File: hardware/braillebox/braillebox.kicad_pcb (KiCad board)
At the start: 2 copper layers, 30 x 30 mm, 1 part, among them U1 XIAO-ESP32-S3-DIP

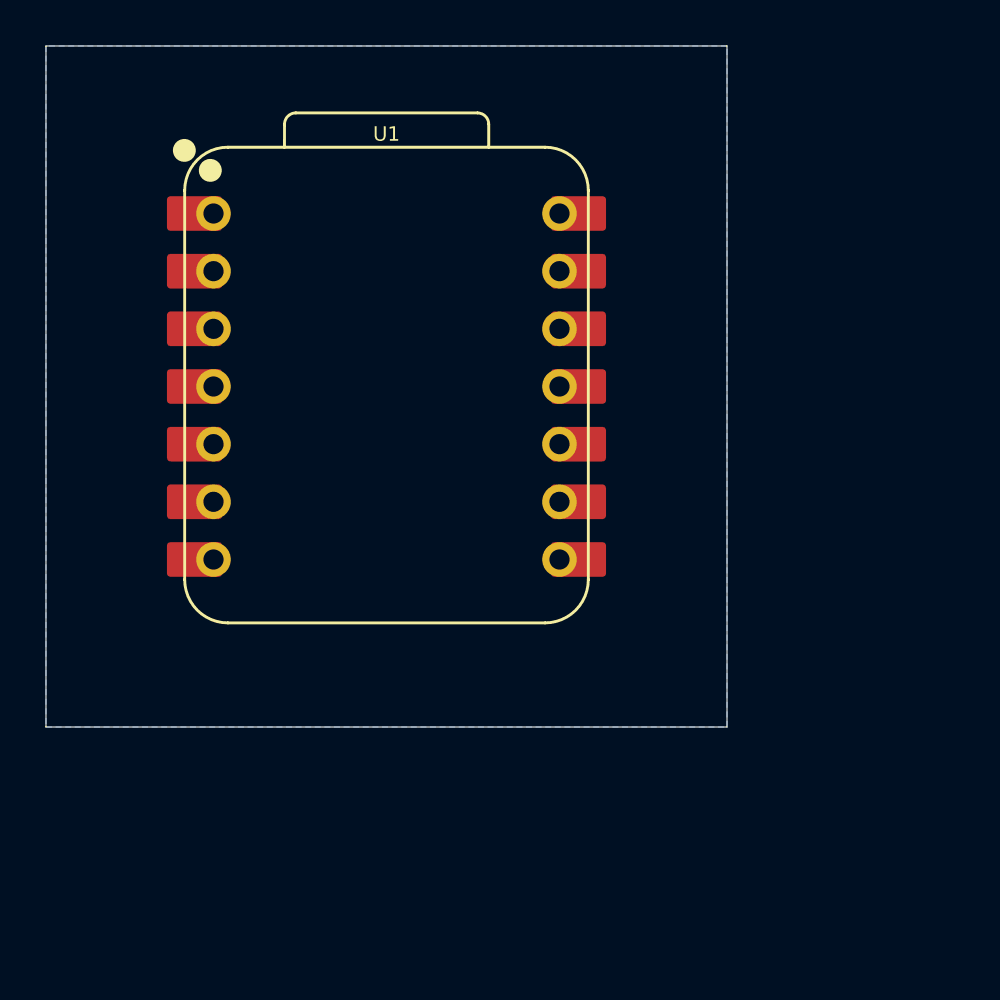
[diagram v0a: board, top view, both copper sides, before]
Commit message: Make circuit
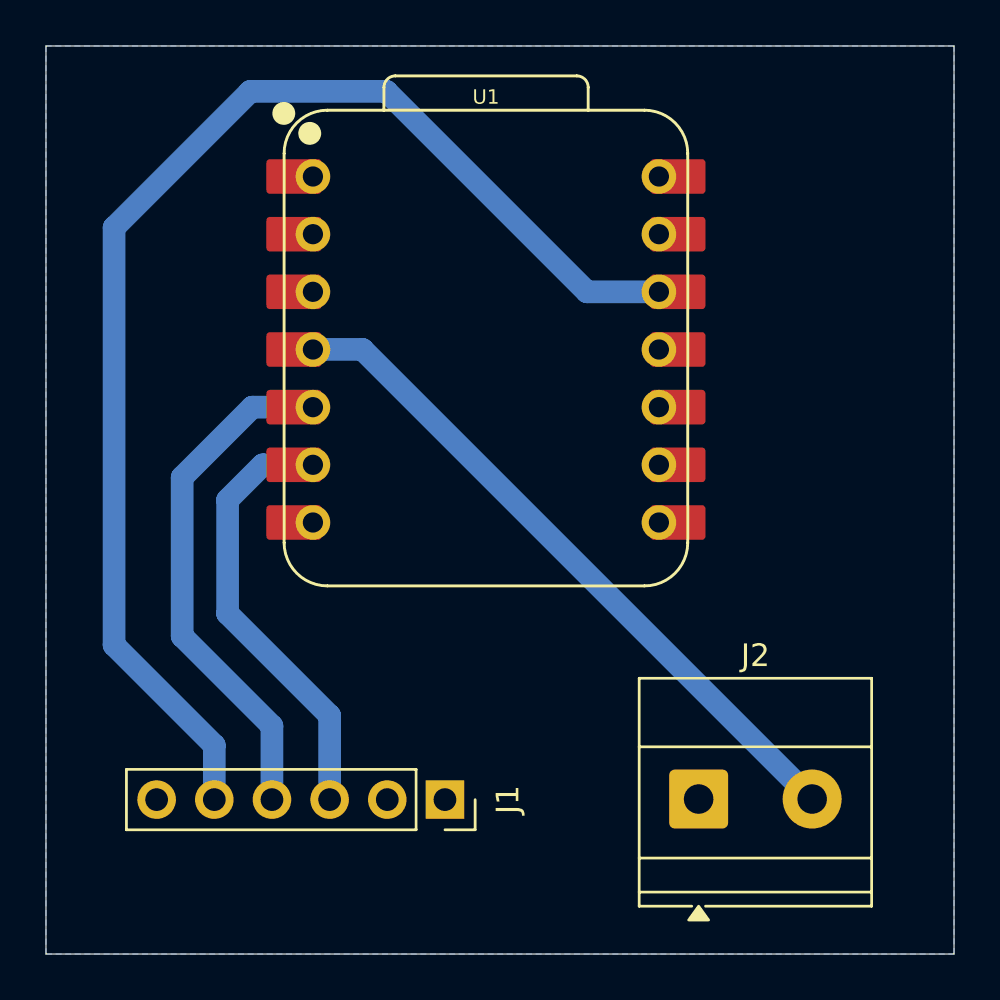
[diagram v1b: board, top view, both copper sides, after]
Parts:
- added J1: PCA9685, Connector_PinSocket_2.54mm:PinSocket_1x06_P2.54mm_Vertical, F.Cu at (67.6, 73.2)
- added J2: Botão, TerminalBlock_Phoenix:TerminalBlock_Phoenix_MKDS-1,5-2_1x02_P5.00mm_Horizontal, F.Cu at (78.8, 73.2)
- moved U1 4.67 mm to (69.4, 53.4)
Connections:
- U1 pad 4: unconnected-(U1-GPIO4_A3_D3-Pad4) -> Net-(J2-Pin_2)
- U1 pad 5: unconnected-(U1-GPIO5_A4_D4_SDA-Pad5) -> Net-(J1-Pin_4)
- U1 pad 6: unconnected-(U1-GPIO6_A5_D5_SCL-Pad6) -> Net-(J1-Pin_3)
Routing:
- net +3.3V: track 0.00 -> 57.2 mm
- net Net-(J2-Pin_2): track 0.00 -> 30.2 mm
- net Net-(J1-Pin_4): track 0.00 -> 22.9 mm
- net Net-(J1-Pin_3): track 0.00 -> 19.5 mm
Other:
- board size 30 x 30 mm -> 40 x 40 mm
